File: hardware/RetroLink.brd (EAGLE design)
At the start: 35.2 x 25.4 mm, 16 parts, among them U1 CH559L, U2 SN74LVC8T245PWR

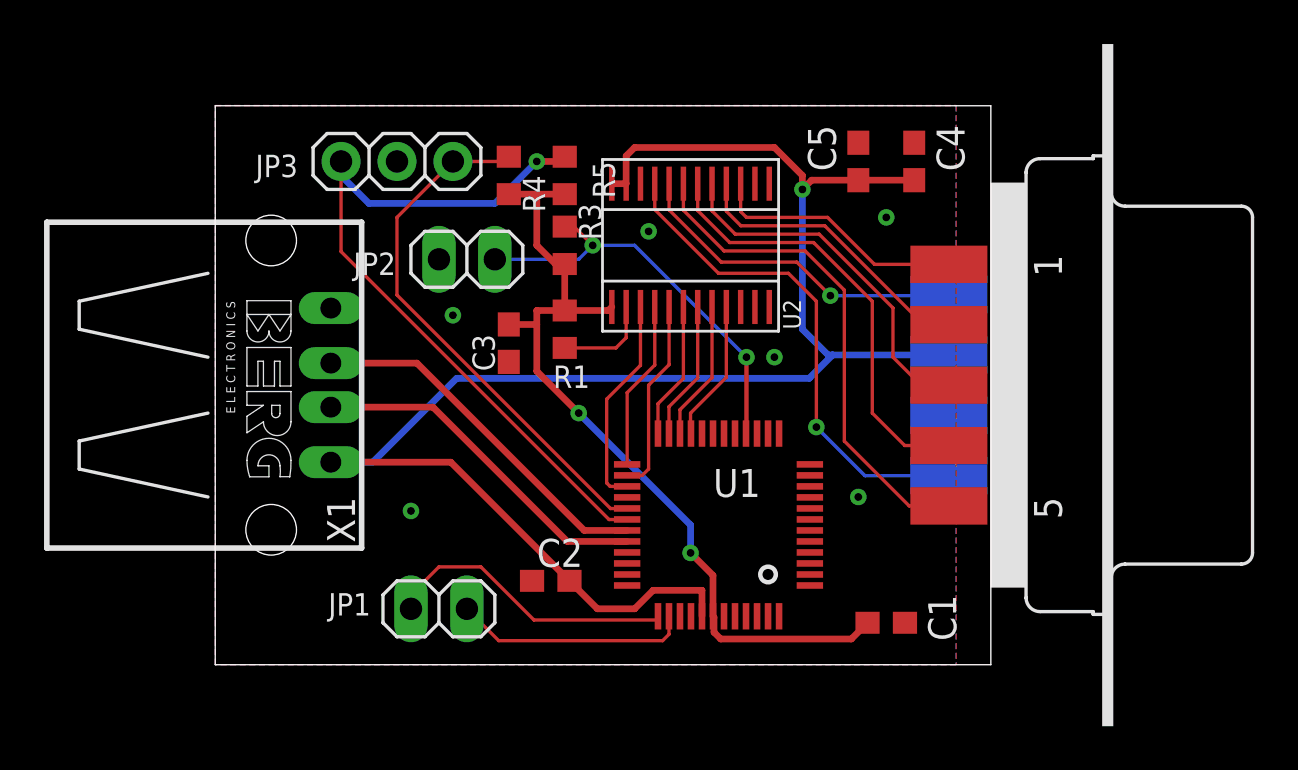
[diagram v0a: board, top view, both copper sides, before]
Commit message: hardware and readme
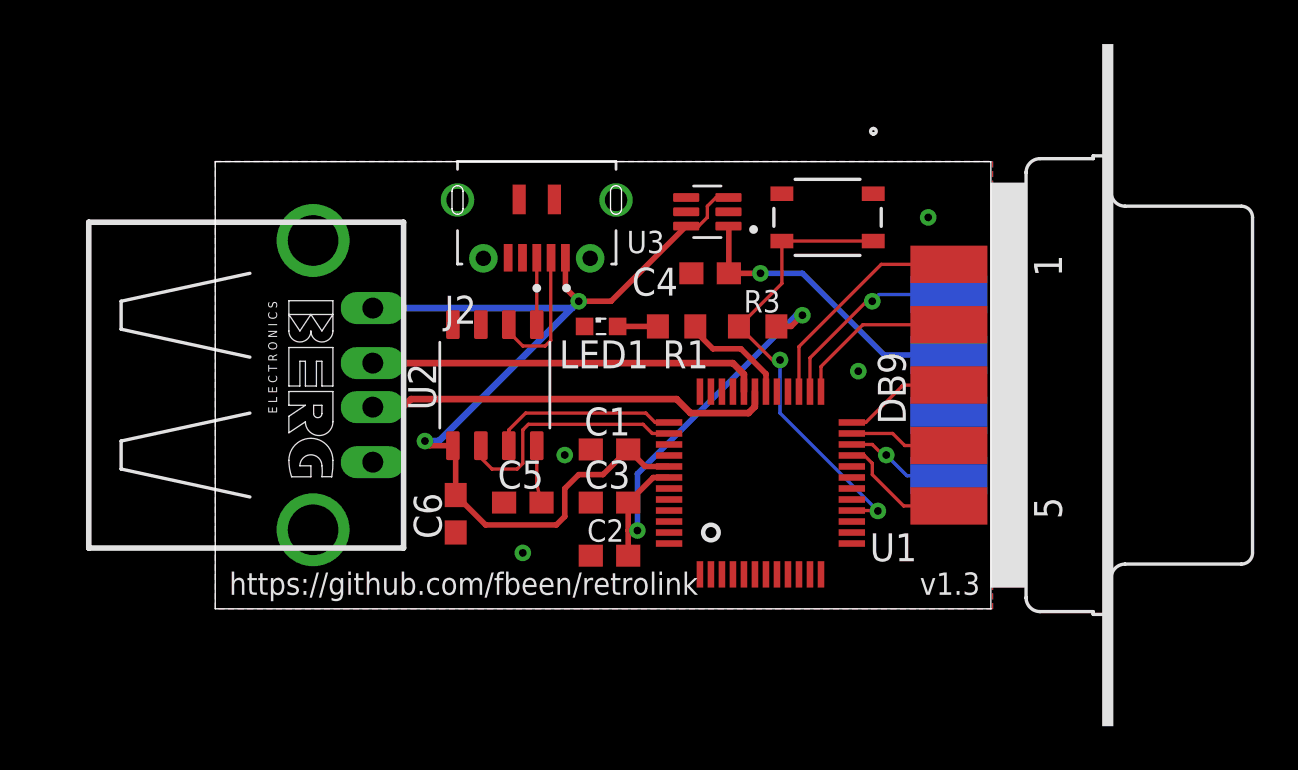
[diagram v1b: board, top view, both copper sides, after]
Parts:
- removed JP1: debug, pinhead:1X02
- removed JP2: PROG, pinhead:1X02
- removed JP3: MODE, pinhead:1X03
- removed R4, R5: 10k, rcl:R0603
- added C6: 100nf, rcl:C0603
- added J2: MICROXNJ, MICROXNJ:SHOUHAN_MICROXNJ
- added LED1: Status, led:SML0603
- added SW1: SKRPABE010, switch:SW4_SKRPABE010_ALPS
- added U3: LM66100DCKR, LM66100DCKR:SOT65P210X110-6N
- C3: value 100nf -> 4.7Uf
- C4: value 100nf -> 10Uf
- C5: value 4.7Uf -> 100nf
- R1: value 10k -> 470
- U2: value SN74LVC8T245PWR -> CH340N; device SN74LVC8T245:TTSOP-24 -> CH340N:SOIC127P600X160-8N
- X1: value (none) -> PN87520-S; device con-berg:PN87520 -> con-berg:PN87520-S
- X3: value (none) -> DB9
- moved C5 21.7 mm to (14.0, 7.37), turned to 0 degrees
- moved C1 14.8 mm to (17.9, 9.78), turned to 0 degrees
- moved U2 10.9 mm to (12.7, 12.7), turned to 270 degrees
- moved C4 10.6 mm to (22.5, 17.8), turned to 0 degrees
- moved R3 9.51 mm to (24.6, 15.4), turned to 0 degrees
- moved C3 8.56 mm to (17.9, 7.37), turned to 0 degrees
- moved R1 5.08 mm to (21.0, 15.4), turned to 0 degrees
- moved C2 2.90 mm to (17.9, 4.95)
- moved U1 2.69 mm to (24.8, 8.26), turned to 90 degrees
- moved X1 1.91 mm to (4.45, 12.7)
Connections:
- removed net N$1: U2.P$15, X3.1
- removed net N$10: R1.1, U2.P$2
- removed net N$2: U2.P$20, X3.6
- removed net N$3: U2.P$21, X3.9
- removed net P2.0: U1.P2.0/A8, U2.P$9
- removed net P2.1: U1.P2.1/MOSI1/A9, U2.P$8
- removed net P2.2: U1.P2.2/MISO1/A10, U2.P$7
- removed net P2.3: U1.P2.3/SCK1/A11, U2.P$6
- removed net P2.4: U1.P2.4/PWM1/A12, U2.P$4
- removed net P2.5: U1.P2.5/TNOW/PWM2/A13/T2EX_/CAP2_, U2.P$5
- removed net P2.6: U1.P2.6/RXD1/A14, U2.P$3
- removed net PROG: JP2.1, R3.1, U1.P4.6/XI/SCS_
- new net 5V_INT: C1.2, C6.2, J2.1, U1.VIN5, U2.5, U3.3, U3.6, X1.1
- new net BTN: R3.1, SW1.3, SW1.4, U1.P4.6/XI/SCS_
- new net CH340V3: C5.2, U2.8
- new net LED: R1.2, U1.P5.4/HM/ALE/XB
- new net MB: U1.P2.0/A8, X3.5
- new net VLED: LED1.A, R1.1
- new net X1: U1.P2.4/PWM1/A12, X3.2
- new net X2: U1.P2.6/RXD1/A14, X3.1
- net DM: now also X1.2; no longer X1.3
- net DP: now also X1.3; no longer X1.2
- net GND: now also C6.1, J2.5, J2.S1, J2.S2, J2.S3, J2.S4, J2.S5, J2.S6, LED1.C, SW1.1, SW1.2, U2.3, U3.2, X1.4, X1.S1, X1.S2; no longer JP2.2, JP3.2, U2.P$11, U2.P$12, U2.P$13, U2.P$22, X1.1
- net LB: now also U1.P2.5/TNOW/PWM2/A13/T2EX_/CAP2_, X3.6; no longer U2.P$17, X3.3
- net N$5: now also J2.2, U2.2; no longer JP3.1, R5.1, U1.P5.4/HM/ALE/XB
- net N$6: now also J2.3, U2.1; no longer JP3.3, R4.1, U1.P5.5/HP/A15/XA
- net RB: now also U1.P2.1/MOSI1/A9, X3.9; no longer U2.P$16, X3.2
- net RXD: now also U2.6; no longer JP1.1
- net TXD: now also U2.7; no longer JP1.2
- net VCC: now also U3.1; no longer C2.2, C5.2, U1.VIN5, U2.P$23, U2.P$24, X1.4
- net VDD33: now also C2.2; no longer C1.2, R1.2, R4.2, R5.2, U2.P$1
- net Y1: now also U1.P2.3/SCK1/A11, X3.3; no longer U2.P$19, X3.5
- net Y2: now also U1.P2.2/MISO1/A10; no longer U2.P$18
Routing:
- net VCC: track 75.9 -> 13.7 mm
- net 5V_INT: track 0.00 -> 46.8 mm, vias 0 -> 2
- net N$5: track 34.3 -> 6.37 mm, vias 1 -> 0
- net N$3: track 22.9 -> 0.00 mm, vias 1 -> 0
- net N$6: track 25.0 -> 3.04 mm
- net BTN: track 0.00 -> 21.2 mm, vias 0 -> 2
- net VDD33: track 38.7 -> 19.6 mm
- net PROG: track 18.9 -> 0.00 mm, vias 2 -> 0
- net Y1: track 22.8 -> 5.11 mm
- net N$2: track 15.5 -> 0.00 mm, vias 1 -> 0
- net Y2: track 20.0 -> 4.64 mm
- net N$1: track 11.7 -> 0.00 mm
- net X2: track 0.00 -> 10.4 mm
- net P2.6: track 9.63 -> 0.00 mm
- net P2.5: track 8.84 -> 0.00 mm
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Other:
- board size 35.2 x 25.4 mm -> 35.2 x 20.3 mm
- board text added: "DB9"
- board text added: "https://github.com/fbeen/retrolink"
- board text added: "v1.3"
